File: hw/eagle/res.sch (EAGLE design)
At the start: 65 parts, among them IC2 7805T, IC3 L272M, IC4 L272M, X5 22-23-2021

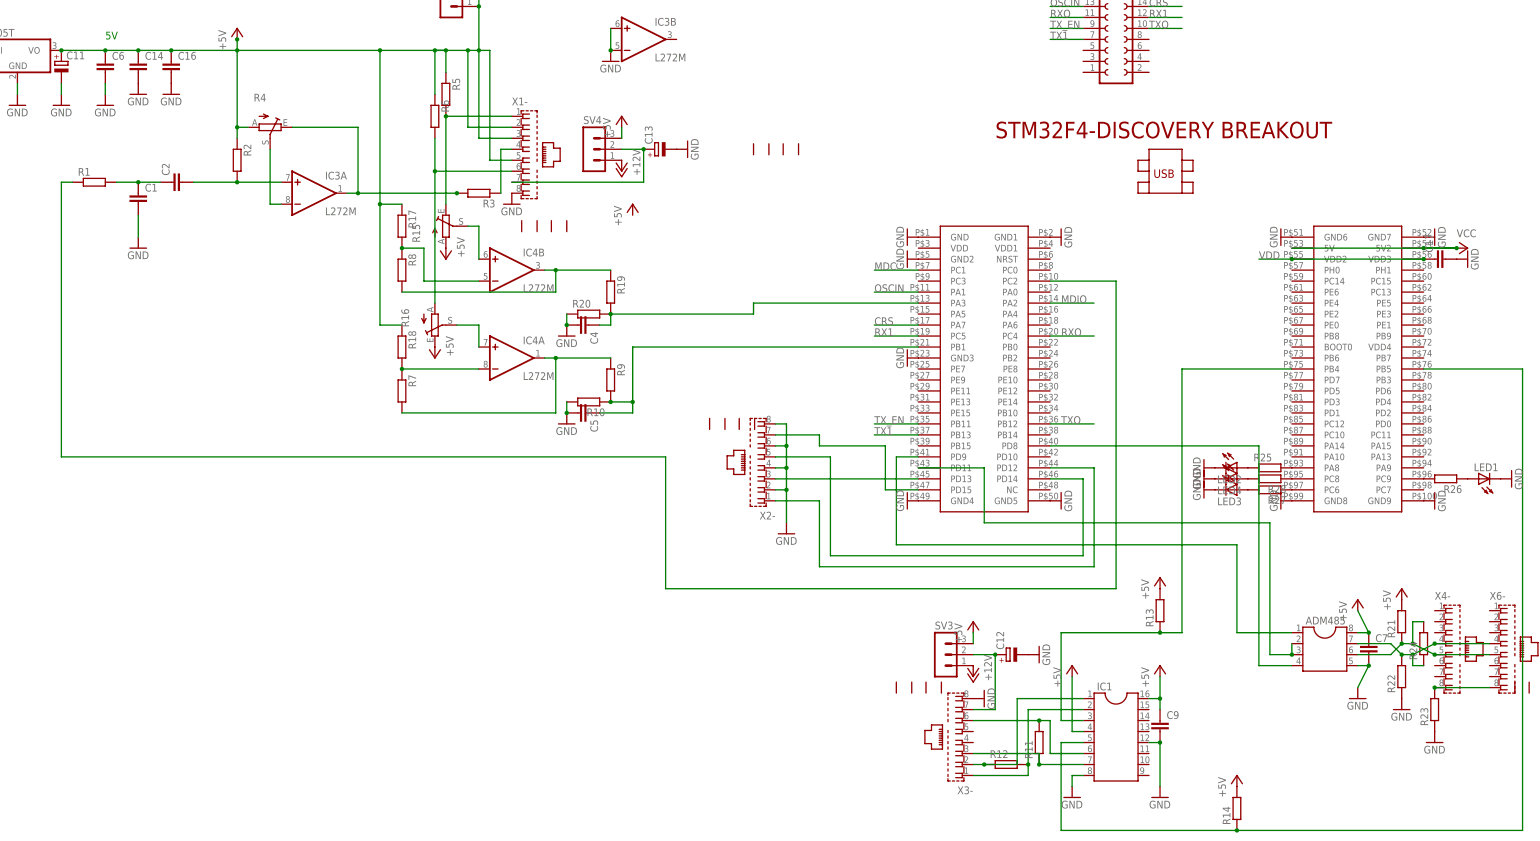
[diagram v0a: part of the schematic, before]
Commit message: bauteilwerte
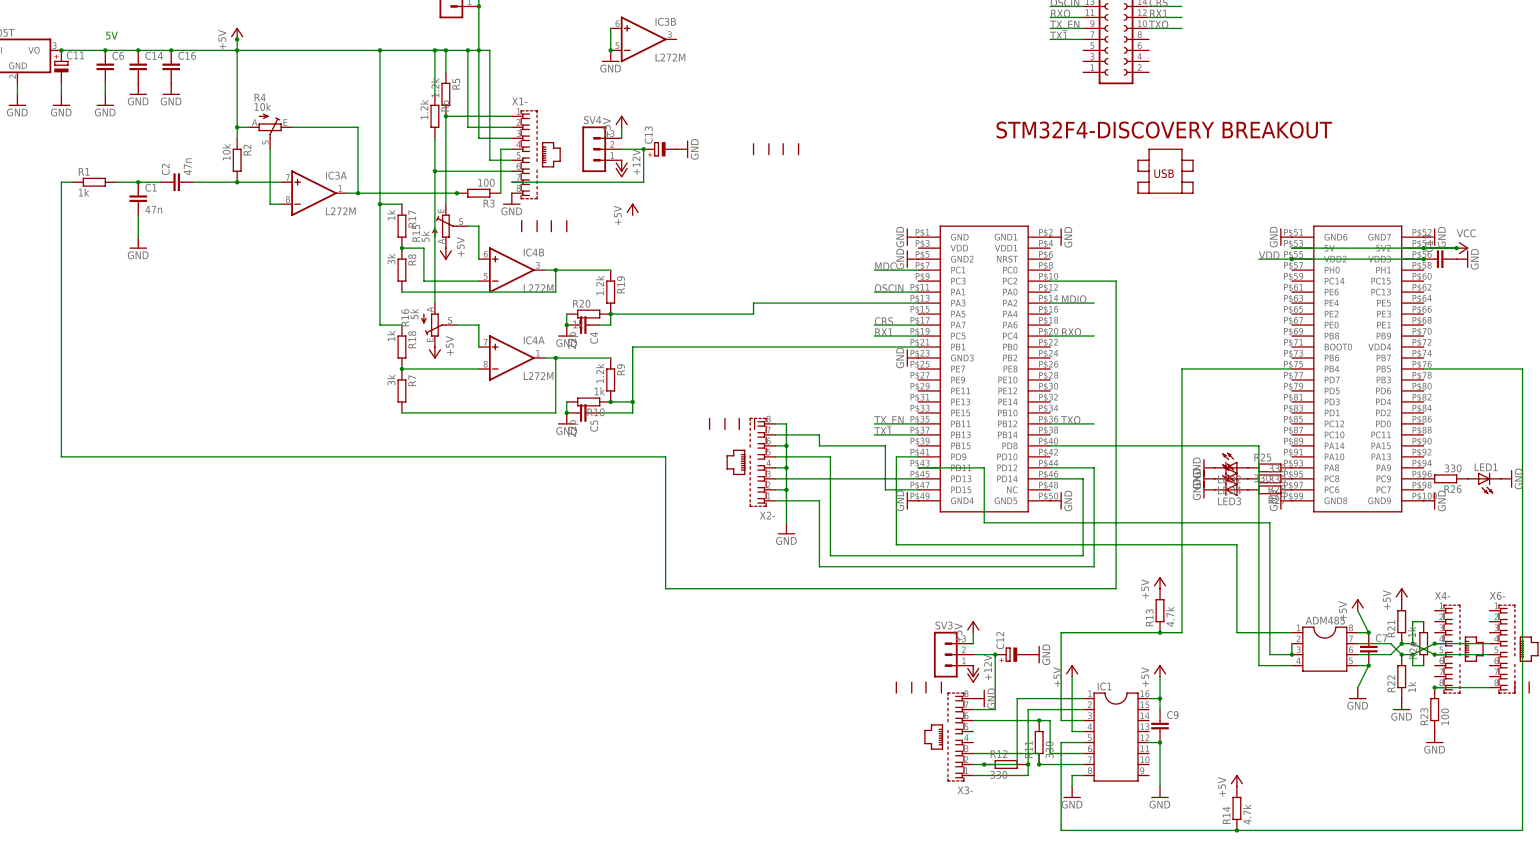
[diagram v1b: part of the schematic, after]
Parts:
- C1, C2: value (none) -> 47n
- C4, C5: value (none) -> 22p
- R1, R10, R17, R18, R20, R21, R22: value (none) -> 1k
- R11, R12, R25, R26, R27, R28: value (none) -> 330
- R13, R14: value (none) -> 4.7k
- R15, R16: value (none) -> 5k
- R19, R5, R6, R9: value (none) -> 1.2k
- R2, R4: value (none) -> 10k
- R23, R3: value (none) -> 100
- R7, R8: value (none) -> 3k
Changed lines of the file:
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@@
 <part name="IC3" library="linear" deviceset="L272" device="M"/>
 <part name="IC4" library="linear" deviceset="L272" device="M"/>
-<part name="R1" library="resistor" deviceset="R-EU_" device="0204/7"/>
-<part name="C1" library="rcl" deviceset="C-EU" device="050-025X075"/>
-<part name="C2" library="rcl" deviceset="C-EU" device="050-025X075"/>
+<part name="R1" library="resistor" deviceset="R-EU_" device="0204/7" value="1k"/>
+<part name="C1" library="rcl" deviceset="C-EU" device="050-025X075" value="47n"/>
+<part name="C2" library="rcl" deviceset="C-EU" device="050-025X075" value="47n"/>
 <part name="C3" library="rcl" deviceset="C-EU" device="050-025X075"/>
 <part name="GND1" library="supply1" deviceset="GND" device=""/>
-<part name="R2" library="resistor" deviceset="R-EU_" device="0204/7"/>
-<part name="R3" library="resistor" deviceset="R-EU_" device="0204/7"/>
-<part name="R4" library="pot" deviceset="TRIM_EU-" device="CA6V"/>
-<part name="R5" library="resistor" deviceset="R-EU_" device="0204/7"/>
-<part name="R6" library="resistor" deviceset="R-EU_" device="0204/7"/>
+<part name="R2" library="resistor" deviceset="R-EU_" device="0204/7" value="10k"/>
+<part name="R3" library="resistor" deviceset="R-EU_" device="0204/7" value="100"/>
+<part name="R4" library="pot" deviceset="TRIM_EU-" device="CA6V" value="10k"/>
+<part name="R5" library="resistor" deviceset="R-EU_" device="0204/7" value="1.2k"/>
+<part name="R6" library="resistor" deviceset="R-EU_" device="0204/7" value="1.2k"/>
 <part name="GND2" library="supply1" deviceset="GND" device=""/>
 <part name="GND3" library="supply1" deviceset="GND" device=""/>
-<part name="C4" library="rcl" deviceset="C-EU" device="050-025X075"/>
-<part name="C5" library="rcl" deviceset="C-EU" device="050-025X075"/>
+<part name="C4" library="rcl" deviceset="C-EU" device="050-025X075" value="22p"/>
+<part name="C5" library="rcl" deviceset="C-EU" device="050-025X075" value="22p"/>
 <part name="GND5" library="supply1" deviceset="GND" device=""/>
 <part name="C6" library="rcl" deviceset="C-EU" device="050-025X075"/>
@@
 <part name="GND19" library="supply1" deviceset="GND" device=""/>
 <part name="X4" library="con-appsys" deviceset="RJ45" device=""/>
-<part name="R11" library="resistor" deviceset="R-EU_" device="0204/7"/>
-<part name="R12" library="resistor" deviceset="R-EU_" device="0204/7"/>
+<part name="R11" library="resistor" deviceset="R-EU_" device="0204/7" value="330"/>
+<part name="R12" library="resistor" deviceset="R-EU_" device="0204/7" value="330"/>
 <part name="P+2" library="supply1" deviceset="VCC" device=""/>
 <part name="C9" library="rcl" deviceset="C-EU" device="050-025X075"/>
@@
 <part name="P+4" library="supply1" deviceset="VCC" device=""/>
 <part name="SV2" library="con-lsta" deviceset="FE10-2W" device=""/>
-<part name="R13" library="resistor" deviceset="R-EU_" device="0204/7"/>
-<part name="R14" library="resistor" deviceset="R-EU_" device="0204/7"/>
+<part name="R13" library="resistor" deviceset="R-EU_" device="0204/7" value="4.7k"/>
+<part name="R14" library="resistor" deviceset="R-EU_" device="0204/7" value="4.7k"/>
 <part name="SV3" library="con-lstb" deviceset="MA03-1" device=""/>
 <part name="P+8" library="supply1" deviceset="+12V" device=""/>
@@
 <part name="P+12" library="supply1" deviceset="+5V" device=""/>
 <part name="GND28" library="supply1" deviceset="GND" device=""/>
-<part name="R15" library="pot" deviceset="TRIM_EU-" device="CA6V"/>
-<part name="R8" library="resistor" deviceset="R-EU_" device="0204/7"/>
-<part name="R17" library="resistor" deviceset="R-EU_" device="0204/7"/>
-<part name="R7" library="resistor" deviceset="R-EU_" device="0204/7"/>
-<part name="R18" library="resistor" deviceset="R-EU_" device="0204/7"/>
-<part name="R16" library="pot" deviceset="TRIM_EU-" device="CA6V"/>
-<part name="R9" library="resistor" deviceset="R-EU_" device="0204/7"/>
-<part name="R10" library="resistor" deviceset="R-EU_" device="0204/7"/>
-<part name="R19" library="resistor" deviceset="R-EU_" device="0204/7"/>
-<part name="R20" library="resistor" deviceset="R-EU_" device="0204/7"/>
+<part name="R15" library="pot" deviceset="TRIM_EU-" device="CA6V" value="5k"/>
+<part name="R8" library="resistor" deviceset="R-EU_" device="0204/7" value="3k"/>
+<part name="R17" library="resistor" deviceset="R-EU_" device="0204/7" value="1k"/>
+<part name="R7" library="resistor" deviceset="R-EU_" device="0204/7" value="3k"/>
+<part name="R18" library="resistor" deviceset="R-EU_" device="0204/7" value="1k"/>
+<part name="R16" library="pot" deviceset="TRIM_EU-" device="CA6V" value="5k"/>
+<part name="R9" library="resistor" deviceset="R-EU_" device="0204/7" value="1.2k"/>
+<part name="R10" library="resistor" deviceset="R-EU_" device="0204/7" value="1k"/>
+<part name="R19" library="resistor" deviceset="R-EU_" device="0204/7" value="1.2k"/>
+<part name="R20" library="resistor" deviceset="R-EU_" device="0204/7" value="1k"/>
 <part name="P+15" library="supply1" deviceset="+5V" device=""/>
 <part name="X5" library="con-molex" deviceset="22-23-2021" device=""/>
@@
 <part name="P+16" library="supply1" deviceset="+5V" device=""/>
 <part name="GND6" library="supply1" deviceset="GND" device=""/>
-<part name="R21" library="resistor" deviceset="R-EU_" device="0204/7"/>
-<part name="R22" library="resistor" deviceset="R-EU_" device="0204/7"/>
-<part name="R23" library="resistor" deviceset="R-EU_" device="0204/7"/>
+<part name="R21" library="resistor" deviceset="R-EU_" device="0204/7" value="1k"/>
+<part name="R22" library="resistor" deviceset="R-EU_" device="0204/7" value="1k"/>
+<part name="R23" library="resistor" deviceset="R-EU_" device="0204/7" value="100"/>
 <part name="R24" library="resistor" deviceset="R-EU_" device="0204/7"/>
 <part name="P+17" library="supply1" deviceset="+5V" device=""/>
@@
 <part name="GND32" library="supply1" deviceset="GND" device=""/>
 <part name="X6" library="con-appsys" deviceset="RJ45" device=""/>
-<part name="R25" library="resistor" deviceset="R-EU_" device="0204/7"/>
-<part name="R26" library="resistor" deviceset="R-EU_" device="0204/7"/>
-<part name="R27" library="resistor" deviceset="R-EU_" device="0204/7"/>
-<part name="R28" library="resistor" deviceset="R-EU_" device="0204/7"/>
+<part name="R25" library="resistor" deviceset="R-EU_" device="0204/7" value="330"/>
+<part name="R26" library="resistor" deviceset="R-EU_" device="0204/7" value="330"/>
+<part name="R27" library="resistor" deviceset="R-EU_" device="0204/7" value="330"/>
+<part name="R28" library="resistor" deviceset="R-EU_" device="0204/7" value="330"/>
 <part name="LED1" library="led" deviceset="LED" device="3MM"/>
 <part name="LED2" library="led" deviceset="LED" device="3MM"/>
